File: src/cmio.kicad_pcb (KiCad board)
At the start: 2 copper layers, 72.4 x 36.8 mm, 37 parts, among them J15 CONN_01X02, J2 BANK0, J4 DSI0, J5 CM3Lite, J6 DSI1, J8 BANK1, J9 Micro_SD_Card_TFP09_2_12B, U1 ISL91107IR, U2 LD3985M18R, U3 LD3985M28R

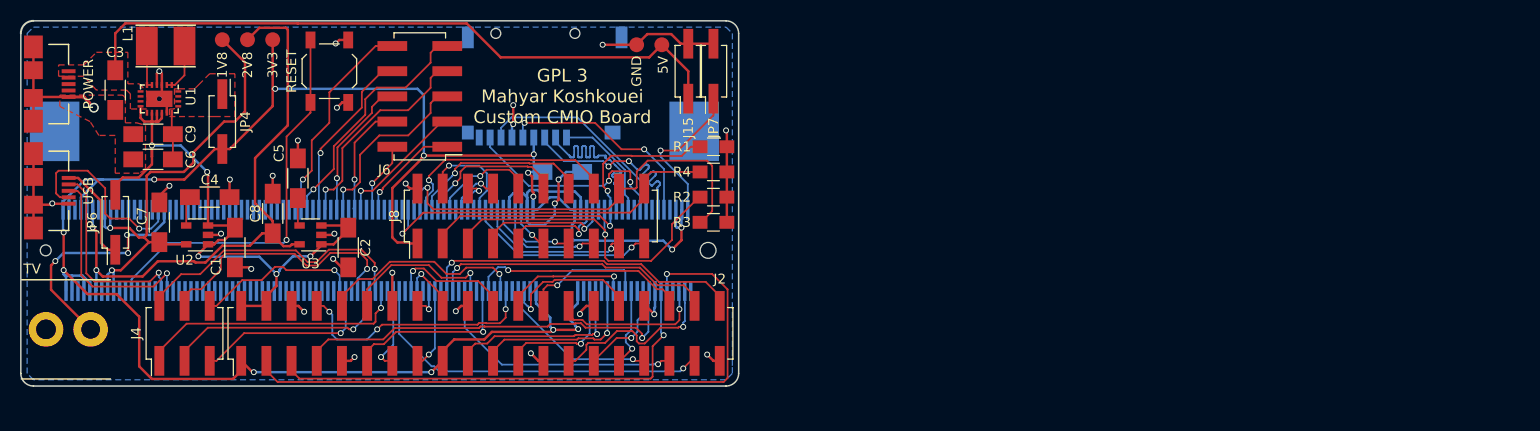
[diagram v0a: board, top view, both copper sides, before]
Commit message: Some changes to old design
Signed-off-by: Mahyar Koshkouei <mk@deltabeard.com>
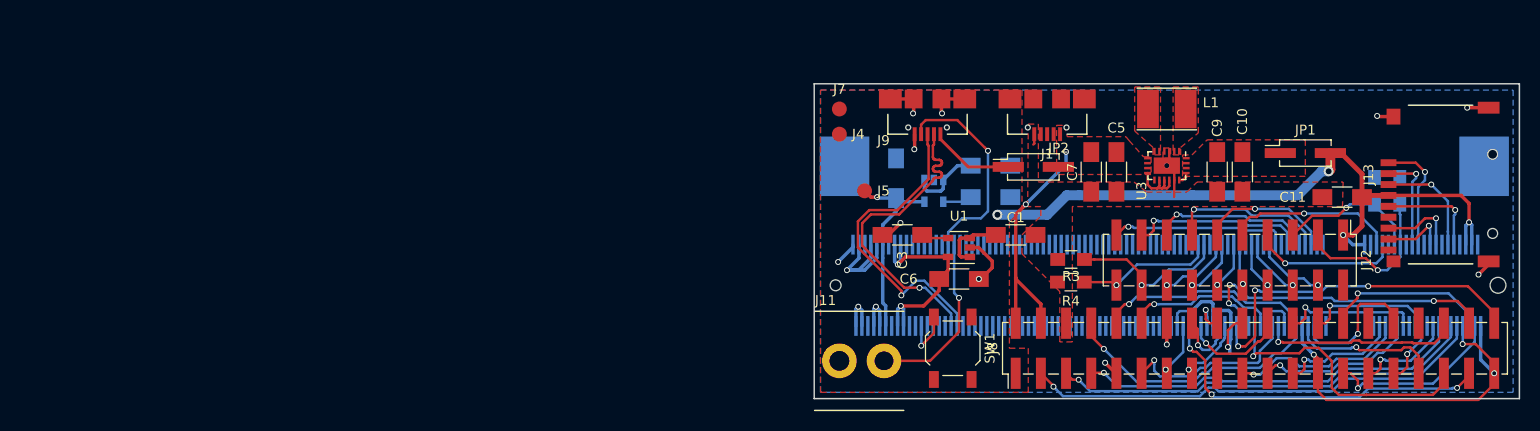
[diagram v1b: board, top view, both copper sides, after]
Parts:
- removed 1V8: TEST_1V8, Measurement_Points:Measurement_Point_Round-SMD-Pad_Small
- removed 2V8: TEST_2V8, Measurement_Points:Measurement_Point_Round-SMD-Pad_Small
- removed 3V3: TEST_3V3, Measurement_Points:Measurement_Point_Round-SMD-Pad_Small
- removed 5V: TEST_5V, Measurement_Points:Measurement_Point_Round-SMD-Pad_Small
- removed GND: TEST_GND, Measurement_Points:Measurement_Point_Round-SMD-Pad_Small
- removed J15: CONN_01X02, Pin_Headers:Pin_Header_Straight_2x01_Pitch2.54mm_SMD
- removed J2: BANK0, Pin_Headers:Pin_Header_Straight_2x20_Pitch2.54mm_SMD
- removed J6: DSI1, Pin_Headers:Pin_Header_Straight_2x05_Pitch2.54mm_SMD
- removed JP4: 3.3 OUT, Pin_Headers:Pin_Header_Straight_2x01_Pitch2.54mm_SMD
- removed JP6: PWRUSB, Pin_Headers:Pin_Header_Straight_2x01_Pitch2.54mm_SMD
- removed JP7: Disable SD Card, Pin_Headers:Pin_Header_Straight_2x01_Pitch2.54mm_SMD
- removed POWER: USB_POWER, foot:Micro_USB_B_10104110_no_holes
- removed RESET: Reset, Buttons_Switches_SMD:SW_SPST_TL3342
- removed TV: TVOUT, foot:RCA_PHONO
- removed USB: USB_OTG, foot:Micro_USB_B_10104110_no_holes
- added C11: 4.7uF, Capacitors_SMD:C_1206_HandSoldering, F.Cu at (208.2, 67.3)
- added J1: USB_POWER, foot:Micro_USB_B_10104110, F.Cu at (178.4, 61.0)
- added J10: CM3Lite, foot:Socket_SODIMM_DDR1-2_TE_1612618, B.Cu at (190.5, 76.2)
- added J11: TVOUT, foot:RCA_PHONO, F.Cu at (157.5, 83.8)
- added J12: BANK1, Pin_Headers:Pin_Header_Straight_2x10_Pitch2.54mm_SMD, F.Cu at (196.8, 73.7)
- added J13: Micro_SD_Card_TFP09_2_12B, foot:TFP09-2-12B, F.Cu at (213.4, 66.0)
- added J7: TEST_GND, Measurement_Points:Measurement_Point_Round-SMD-Pad_Small, F.Cu at (157.5, 58.4)
- added JP1: 3.3 OUT, Pin_Headers:Pin_Header_Straight_2x01_Pitch2.54mm_SMD, F.Cu at (204.5, 62.9)
- added JP2: PWRUSB, Pin_Headers:Pin_Header_Straight_2x01_Pitch2.54mm_SMD, F.Cu at (177.0, 64.3)
- added SW1: Reset, Buttons_Switches_SMD:SW_SPST_TL3342, F.Cu at (168.9, 82.5)
- C10: value 4.7uF -> 22uF; moved to F.Cu
- C2, C4, C8, R1, R2: moved to B.Cu
- C3: value 22uF -> 10nF
- C5: value 10nF -> 1uF
- C6: value 22uF -> 1uF
- C7: value 1uF -> 22uF
- J4: value DSI0 -> TEST_3V3; footprint Pin_Headers:Pin_Header_Straight_2x03_Pitch2.54mm_SMD -> Measurement_Points:Measurement_Point_Round-SMD-Pad_Small
- J5: value CM3Lite -> TEST_2V8; footprint foot:Socket_SODIMM_DDR1-2_TE_1612618 -> Measurement_Points:Measurement_Point_Round-SMD-Pad_Small; moved to F.Cu
- J8: value BANK1 -> BANK0; footprint Pin_Headers:Pin_Header_Straight_2x10_Pitch2.54mm_SMD -> Pin_Headers:Pin_Header_Straight_2x20_Pitch2.54mm_SMD
- J9: value Micro_SD_Card_TFP09_2_12B -> USB_OTG; footprint foot:TFP09-2-12B -> foot:Micro_USB_B_10104110; moved to F.Cu
- U1: value ISL91107IR -> LD3985M18R; footprint foot:20_TQFP -> TO_SOT_Packages_SMD:SOT-23-5
- U2: value LD3985M18R -> LD3985M28R; moved to B.Cu
- U3: value LD3985M28R -> ISL91107IR; footprint TO_SOT_Packages_SMD:SOT-23-5 -> foot:20_TQFP
- moved C9 107.4 mm to (195.6, 64.8), turned to 90 degrees
- moved L1 101.2 mm to (190.5, 58.4)
- moved C7 94.1 mm to (182.9, 64.8), turned to 270 degrees
- moved U3 86.6 mm to (190.5, 64.1), turned to 270 degrees
- moved C5 82.6 mm to (185.4, 64.8), turned to 270 degrees
- moved C6 82.2 mm to (169.5, 75.6)
- moved U1 82.0 mm to (169.5, 72.4), turned to 180 degrees
- moved C3 80.7 mm to (163.8, 71.1), turned to 180 degrees
- moved C1 78.8 mm to (175.3, 71.1), turned to 0 degrees
- moved C4 78.7 mm to (172.7, 67.3)
- moved U2 74.4 mm to (167.0, 66.7), turned to 270 degrees
- moved J8 74.2 mm to (199.4, 82.5)
- moved R1 69.4 mm to (214.0, 66.7), turned to 90 degrees
- moved J4 69.0 mm to (157.5, 61.0), turned to 0 degrees
- moved C10 68.6 mm to (198.1, 64.8), turned to 90 degrees
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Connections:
- C1 pad 1: +5V -> +3V3
- C10 pad 1: +3V3 -> GND
- C10 pad 2: GND -> Net-(C10-Pad2)
- C2 pad 1: +5V -> +3V3
- C3 pad 1: +5V -> Net-(C3-Pad1)
- C5 pad 1: Net-(C5-Pad1) -> +5V
- C6 pad 1: GND -> +1V8
- C6 pad 2: Net-(C6-Pad2) -> GND
- C7 pad 1: +1V8 -> +5V
- C9 pad 2: Net-(C6-Pad2) -> Net-(C10-Pad2)
- J4 pad 1: /DSI0_0 -> +3V3
- J5 pad 1: GND -> +2V8
- J8 pad 10: /BCM_40 -> /BCM_15
- J8 pad 11: /BCM_32 -> /BCM_17
- J8 pad 12: /BCM_41 -> /BCM_18
- J8 pad 13: /BCM_33 -> /BCM_27
- J8 pad 14: /BCM_42 -> GND
- J8 pad 15: /BCM_34 -> /BCM_22
- J8 pad 16: /BCM_43 -> /BCM_23
- J8 pad 17: /BCM_35 -> +3V3
- J8 pad 18: /BCM_44 -> /BCM_24
- J8 pad 19: /BCM_36 -> /BCM_10
- J8 pad 2: GND -> +5V
- J8 pad 20: /BCM_45 -> GND
- J8 pad 3: /BCM_28 -> /BCM_2
- J8 pad 4: /BCM_37 -> +5V
- J8 pad 5: /BCM_29 -> /BCM_3
- J8 pad 6: /BCM_38 -> GND
- J8 pad 7: /BCM_30 -> /BCM_4
- J8 pad 8: /BCM_39 -> /BCM_14
- J8 pad 9: /BCM_31 -> GND
- J9 pad 1: DAT2 -> Net-(J9-Pad1)
- J9 pad 2: DAT3 -> /D-
- J9 pad 3: CMD -> /D+
- J9 pad 4: +3V3 -> OTDIG
- J9 pad 5: CLK -> GND
- U1 pad 1: Net-(L1-Pad1) -> +3V3
- U1 pad 2: Net-(L1-Pad1) -> GND
- U1 pad 3: GND -> +3V3
- U1 pad 4: GND -> Net-(C3-Pad1)
- U1 pad 5: Net-(L1-Pad2) -> +1V8
- U2 pad 1: +5V -> +3V3
- U2 pad 3: +5V -> +3V3
- U2 pad 5: +1V8 -> +2V8
- U3 pad 1: +5V -> Net-(L1-Pad1)
- U3 pad 2: GND -> Net-(L1-Pad1)
- U3 pad 3: +5V -> GND
- U3 pad 4: Net-(C5-Pad1) -> GND
- U3 pad 5: +2V8 -> Net-(L1-Pad2)
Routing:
- net +3V3: track 208.1 -> 105.8 mm, vias 14 -> 8
- net +5V: track 132.1 -> 31.1 mm, vias 5 -> 2
- net Net-(J5-Pad177): track 39.6 -> 0.00 mm, vias 1 -> 0
- net +2V8: track 58.9 -> 20.1 mm, vias 2 -> 1
- net /DSI0_1: track 29.1 -> 0.00 mm, vias 1 -> 0
- net /DSI0_0: track 27.4 -> 0.00 mm, vias 1 -> 0
- net +1V8: track 49.6 -> 22.2 mm
- net /BCM_44: track 43.5 -> 16.2 mm
- net /DSI0_3: track 26.7 -> 0.00 mm, vias 1 -> 0
- net /DSI1_8: track 24.7 -> 0.00 mm, vias 1 -> 0
- net TVDAC: track 23.8 -> 0.00 mm, vias 3 -> 0
- net /DSI0_2: track 23.4 -> 0.00 mm, vias 1 -> 0
- net /DSI1_6: track 21.8 -> 0.00 mm, vias 1 -> 0
- net /BCM_45: track 36.4 -> 14.9 mm
- net /DSI1_9: track 21.3 -> 0.00 mm, vias 1 -> 0
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- added copper zone on F.Cu, net +3V3
- added copper zone on F.Cu, net Net-(C10-Pad2)
- added copper zone on F.Cu, net Net-(L1-Pad1)
- added copper zone on F.Cu, net Net-(L1-Pad2)
- removed copper zone on F.Cu, net Net-(C6-Pad2)
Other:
- board size 72.4 x 36.8 mm -> 71.1 x 31.7 mm
- net class Default: clearance 0.16 -> 0; trace_width 0.18 -> 0.25
- net class PWR: clearance 0.2 -> 0.25; trace_width 0.25 -> 0.35
- rule trace_clearance: 0.16 -> 0
- rule trace_min: 0.15 -> 0.2
- rule via_min_size: 0.5 -> 0.6
- board text removed: "GPL 3 Mahyar Koshkouei Custom CMIO Board"
